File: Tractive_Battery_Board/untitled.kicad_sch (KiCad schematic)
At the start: 2 parts, among them J9 Current Sensor, U1 MCP6004

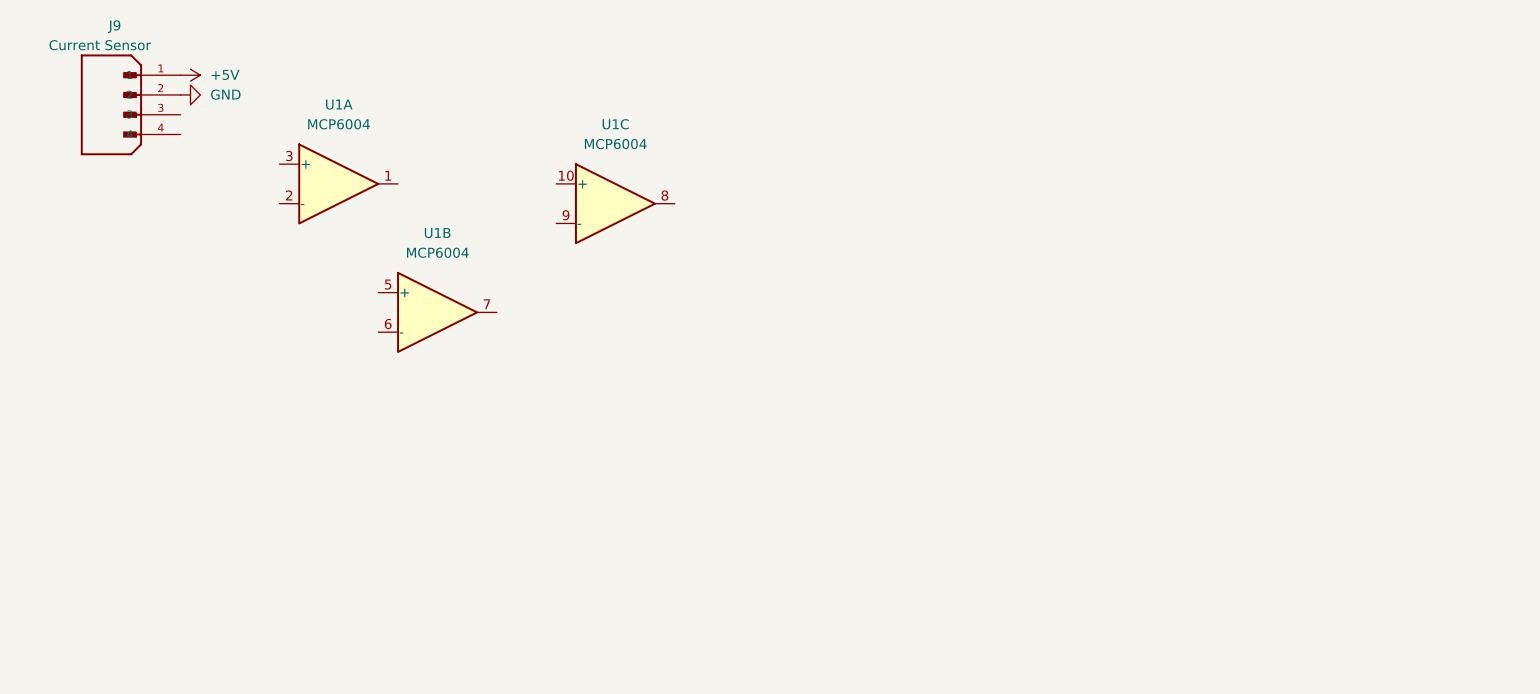
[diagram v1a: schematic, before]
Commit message: Current Sensor
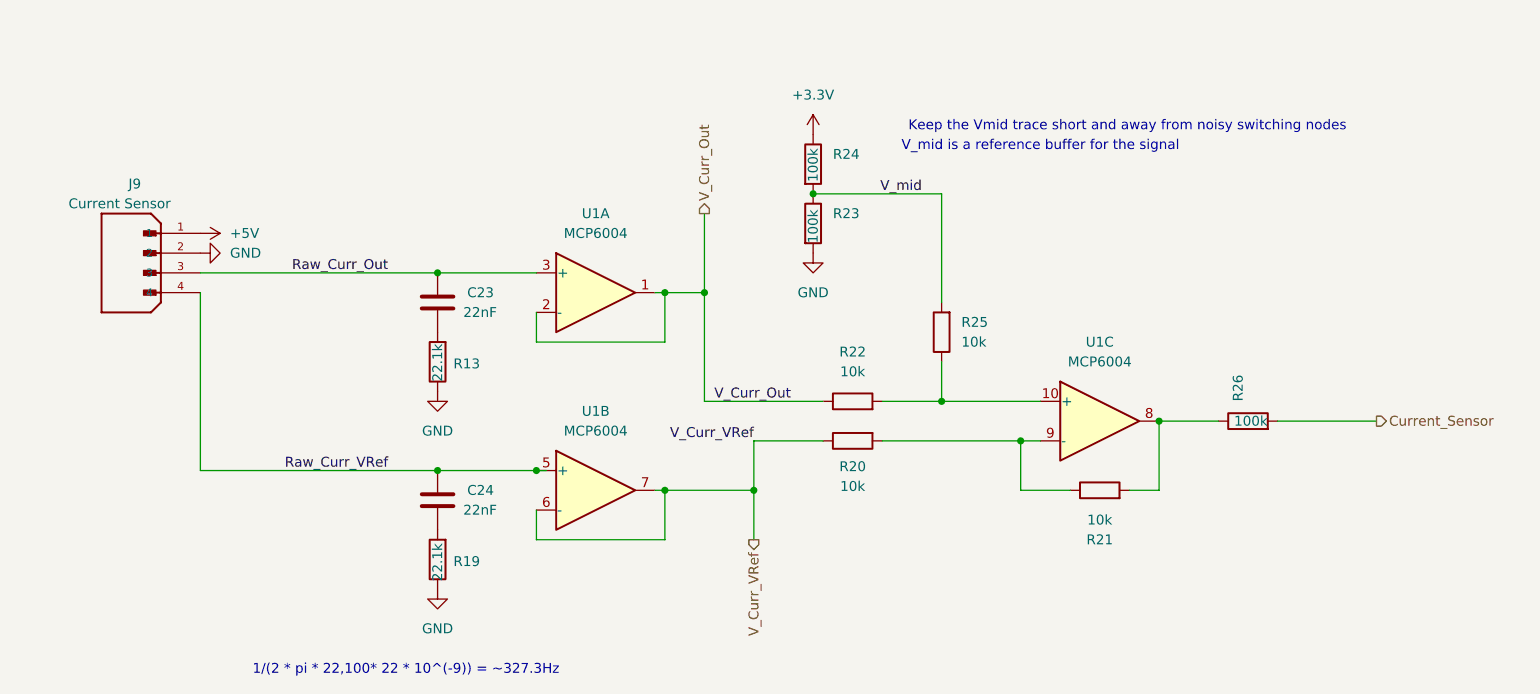
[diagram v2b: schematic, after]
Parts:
- added C23, C24: 22nF, symbol Device:C
- added R13, R19: 22.1k, symbol Device:R
- added R20, R21, R22, R25: 10k, symbol Device:R
- added R23, R24, R26: 100k, symbol Device:R
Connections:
- net GND: now also R13.1, R19.1, R23.2
- net Raw_Curr_Out: now reaches J9.3
- net Raw_Curr_Out: now also U1.3 (+), C23.1
- net Raw_Curr_VRef: now reaches J9.4
- net Raw_Curr_VRef: now also U1.5 (+), C24.1
- net at U1.10 (+): now also R22.2, R25.1
- net at U1.8: now also R21.2, R26.1
- net at U1.9 (-): now also R20.2, R21.1
- net V_Curr_VRef: now reaches U1.6 (-)
- net V_Curr_VRef: now also U1.7, R20.1
- net V_Curr_Out: now reaches U1.1
- net V_Curr_Out: now also U1.2 (-), R22.1
- new net: C23.2, R13.2
- new net: C24.2, R19.2
- new net +3.3V: R24.1
- new net Current_Sensor: R26.2
- new net V_mid: R23.1, R24.2, R25.2
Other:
- note added: "1/(2 * pi * 22,100* 22 * 10^(-9)) = ~327.3Hz"
- note added: "Keep the Vmid trace short and away from noisy switching nodes"
- note added: "V_mid is a reference buffer for the signal"
- moved on the sheet: J9, U1A, U1B, U1C
